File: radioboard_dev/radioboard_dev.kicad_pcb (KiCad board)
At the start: 2 copper layers, 98 parts, among them J1 Conn_01x02, J2 Conn_01x02, J3 Conn_01x04, J4 Conn_01x04, J5 Conn_01x04, J6 Conn_01x04, J9 Conn_01x04, U1 TPS22917DBVR, U10 STM32WL55CCUx, U11 MAX17048G_T10, U12 TPS73733QDRBRQ1, U13 ACS722LLCTR-05AB-T, U2 SAM-M10Q-00B, U5 MCP73831T-2ACI_OT, U8 BGS13SN8E6327XTSA1, Y1 ECS-TXO-25CSMV-320-DY-TR

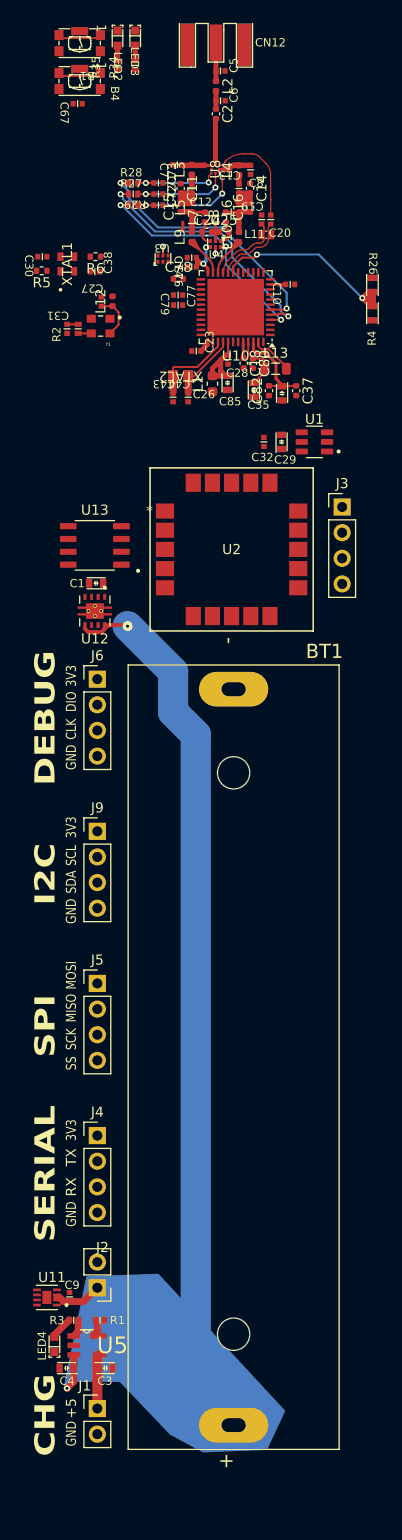
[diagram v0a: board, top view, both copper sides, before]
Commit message: almost done!!!
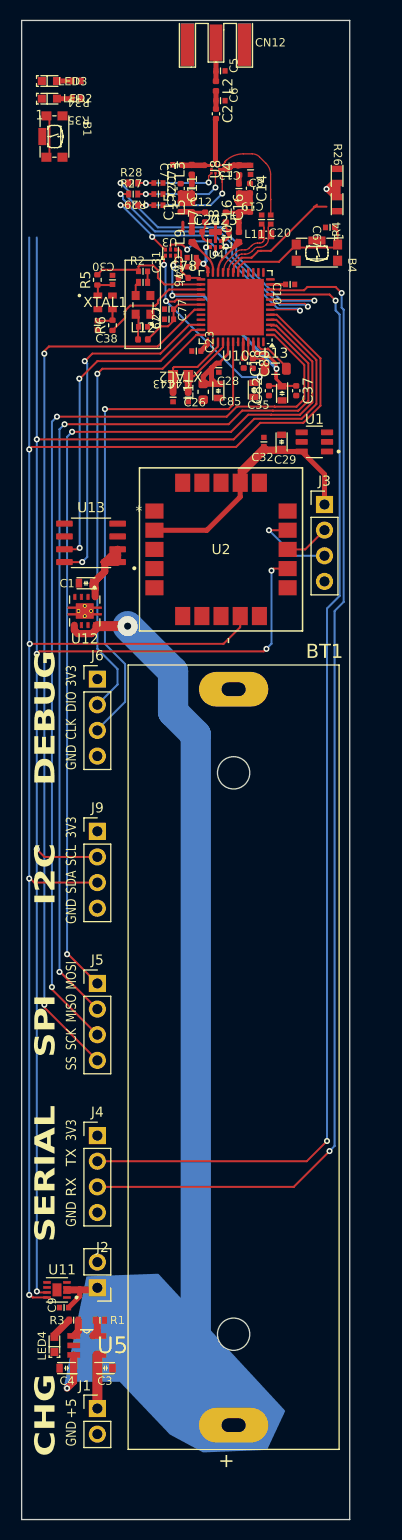
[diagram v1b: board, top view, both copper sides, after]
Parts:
- moved B4 29.0 mm to (51.2, 48.5)
- moved C67 27.8 mm to (52.5, 46.0)
- moved R26 11.4 mm to (53.2, 40.9)
- moved R4 11.4 mm to (53.2, 43.7)
- moved B1 9.58 mm to (25.2, 37.0), turned to 90 degrees
- moved LED3 9.50 mm to (24.8, 31.5), turned to 180 degrees
- moved C31 9.44 mm to (34.0, 50.4), turned to 180 degrees
- moved LED2 9.03 mm to (24.8, 33.2), turned to 180 degrees
- moved R2 7.90 mm to (34.0, 51.5), turned to 0 degrees
- moved C30 7.32 mm to (31.0, 51.2), turned to -90 degrees
- moved R6 7.01 mm to (31.0, 55.7), turned to 90 degrees
- moved R34 6.00 mm to (27.4, 31.5), turned to 180 degrees
- moved R5 5.58 mm to (29.5, 51.2), turned to 90 degrees
- moved XTAL1 5.34 mm to (30.3, 53.4), turned to 0 degrees
- moved C38 5.31 mm to (29.5, 55.7), turned to 90 degrees
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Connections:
- U10 pad 14: unconnected-(U10-PA6-Pad14) -> BUT1
- U10 pad 15: BUT1 -> unconnected-(U10-PA7-Pad15)
- U10 pad 16: GPSPOW -> unconnected-(U10-PA8-Pad16)
- U10 pad 17: SCL -> unconnected-(U10-PA9-Pad17)
- U10 pad 33: SDA -> unconnected-(U10-PA10-Pad33)
- U10 pad 4: /microcontroller_RF/FE_CTRL1 -> SCL
- U10 pad 43: unconnected-(U10-PA15-Pad43) -> GPSPOW
- U10 pad 5: /microcontroller_RF/FE_CTRL2 -> SDA
- U10 pad 6: /microcontroller_RF/FE_CTRL3 -> /microcontroller_RF/FE_CTRL1
- U10 pad 7: unconnected-(U10-PA0-Pad7) -> /microcontroller_RF/FE_CTRL2
- U10 pad 8: unconnected-(U10-PA1-Pad8) -> /microcontroller_RF/FE_CTRL3
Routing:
- net LPUART1_RX: track 0.00 -> 117.6 mm, vias 0 -> 2
- net LPUART1_TX: track 0.00 -> 114.2 mm, vias 0 -> 2
- net SPI1_SCK: track 0.00 -> 96.5 mm, vias 0 -> 2
- net SPI1_MISO: track 0.00 -> 93.7 mm, vias 0 -> 2
- net SPI1_MOSI: track 0.00 -> 90.9 mm, vias 0 -> 2
- net SPI1_NSS: track 0.00 -> 89.6 mm, vias 0 -> 2
- net SCL: track 0.00 -> 79.7 mm, vias 0 -> 6
- net SDA: track 0.00 -> 74.1 mm, vias 0 -> 4
- net SWCLK: track 0.00 -> 52.9 mm, vias 0 -> 1
- net SWDIO: track 0.00 -> 46.3 mm, vias 0 -> 1
- net VCURR: track 0.00 -> 35.0 mm, vias 0 -> 2
- net VGPS: track 0.00 -> 33.7 mm
- net CURROUT: track 0.00 -> 32.4 mm, vias 0 -> 2
- net VDDRF1V55: track 5.79 -> 26.4 mm, vias 0 -> 3
- net VDDRF: track 9.13 -> 29.6 mm, vias 0 -> 3
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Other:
- board outline added: 32.5 x 148.5 mm
